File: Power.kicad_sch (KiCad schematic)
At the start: 48 parts, among them SW901 DP3T, U901 BQ24075, U902 TPS7A0533PDBV, U903 LP5907MFX-3.3

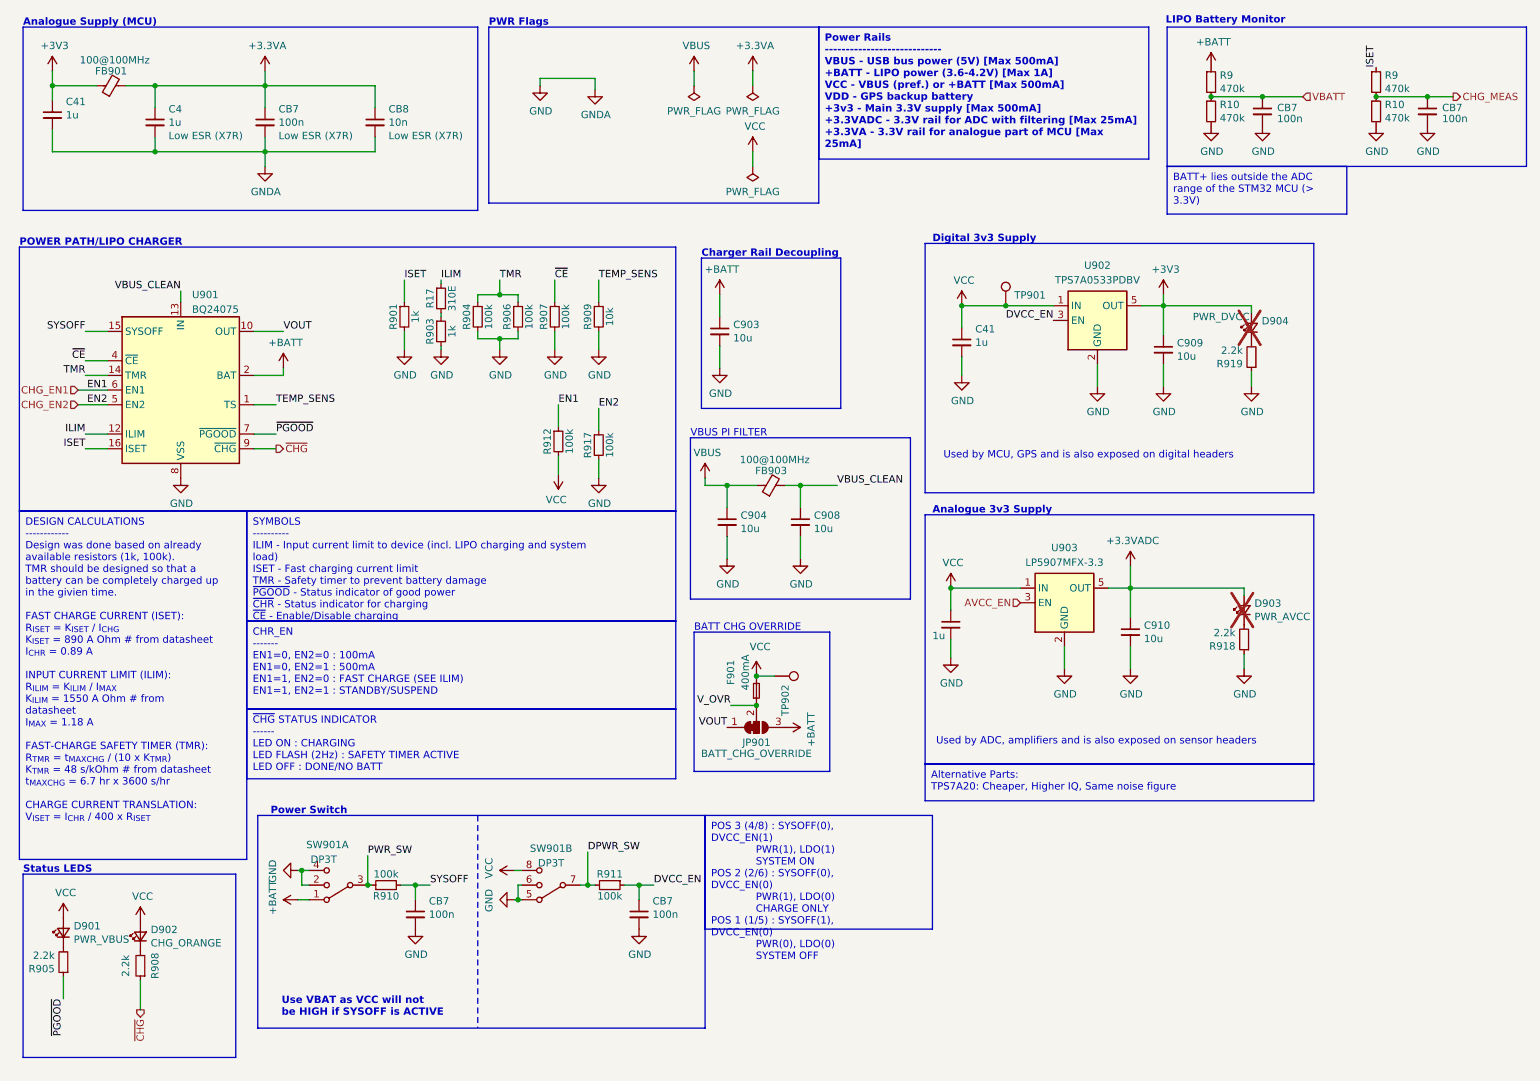
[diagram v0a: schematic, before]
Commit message: (sch) update annotations
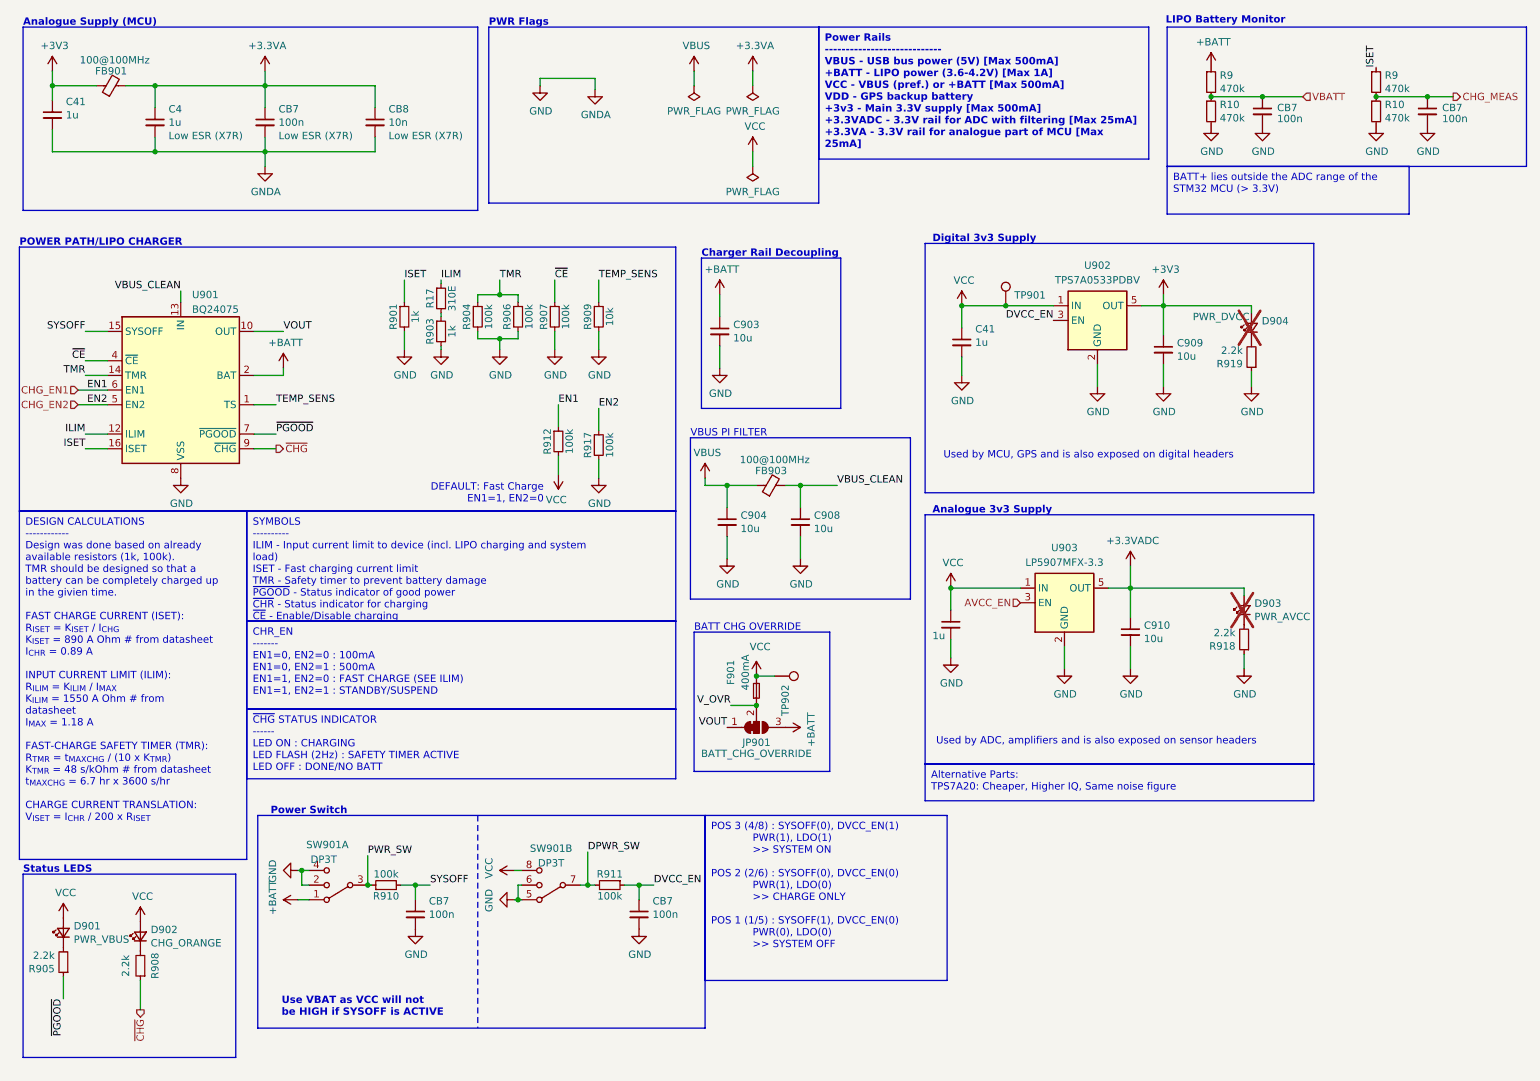
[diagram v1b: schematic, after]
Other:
- note added: "DEFAULT: Fast Charge EN1=1, EN2=0"
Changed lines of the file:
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@@
     (effects (font (size 1.27 1.27)) (justify left top))
   )
-  (text_box "DESIGN CALCULATIONS\n------------\nDesign was done based on already available resistors (1k, 100k).\nTMR should be designed so that a battery can be completely charged up in the givien time.\n\nFAST CHARGE CURRENT (ISET):\nR_{ISET} = K_{ISET} / I_{CHG}\nK_{ISET} = 890 A Ohm # from datasheet\nI_{CHR} = 0.89 A\n\nINPUT CURRENT LIMIT (ILIM):\nR_{ILIM} = K_{ILIM} / I_{MAX}\nK_{ILIM} = 1550 A Ohm # from datasheet\nI_{MAX} = 1.18 A\n\nFAST-CHARGE SAFETY TIMER (TMR):\nR_{TMR} = t_{MAXCHG} / (10 x K_{TMR})\nK_{TMR} = 48 s/kOhm # from datasheet\nt_{MAXCHG} = 6.7 hr x 3600 s/hr\n\nCHARGE CURRENT TRANSLATION:\nV_{ISET} = I_{CHR} / 400 x R_{ISET}"
+  (text_box "DESIGN CALCULATIONS\n------------\nDesign was done based on already available resistors (1k, 100k).\nTMR should be designed so that a battery can be completely charged up in the givien time.\n\nFAST CHARGE CURRENT (ISET):\nR_{ISET} = K_{ISET} / I_{CHG}\nK_{ISET} = 890 A Ohm # from datasheet\nI_{CHR} = 0.89 A\n\nINPUT CURRENT LIMIT (ILIM):\nR_{ILIM} = K_{ILIM} / I_{MAX}\nK_{ILIM} = 1550 A Ohm # from datasheet\nI_{MAX} = 1.18 A\n\nFAST-CHARGE SAFETY TIMER (TMR):\nR_{TMR} = t_{MAXCHG} / (10 x K_{TMR})\nK_{TMR} = 48 s/kOhm # from datasheet\nt_{MAXCHG} = 6.7 hr x 3600 s/hr\n\nCHARGE CURRENT TRANSLATION:\nV_{ISET} = I_{CHR} / 200 x R_{ISET}"
     (at 14.605 100.33 0) (size 39.37 60.325)
     (stroke (width 0) (type default))
@@
     (effects (font (size 1.27 1.27)) (justify left top))
   )
-  (text_box "POS 3 (4/8) : SYSOFF(0), DVCC_EN(1)\n			  PWR(1), LDO(1)\n			  SYSTEM ON\nPOS 2 (2/6) : SYSOFF(0), DVCC_EN(0)\n			  PWR(1), LDO(0)\n			  CHARGE ONLY\nPOS 1 (1/5) : SYSOFF(1), DVCC_EN(0)\n			  PWR(0), LDO(0)\n			  SYSTEM OFF"
-    (at 133.35 153.035 0) (size 39.37 19.685)
+  (text_box "POS 3 (4/8) : SYSOFF(0), DVCC_EN(1)\n			 PWR(1), LDO(1)\n			 >> SYSTEM ON\n\nPOS 2 (2/6) : SYSOFF(0), DVCC_EN(0)\n			 PWR(1), LDO(0)\n			 >> CHARGE ONLY\n\nPOS 1 (1/5) : SYSOFF(1), DVCC_EN(0)\n			 PWR(0), LDO(0)\n			 >> SYSTEM OFF"
+    (at 133.35 153.035 0) (size 41.91 28.575)
     (stroke (width 0) (type default))
     (fill (type none))
@@
   )
   (text_box "BATT+ lies outside the ADC range of the STM32 MCU (> 3.3V)"
-    (at 213.36 40.64 0) (size 31.115 8.255)
+    (at 213.36 40.64 0) (size 41.91 8.255)
     (stroke (width 0) (type default))
     (fill (type none))
@@
     (effects (font (size 1.27 1.27) (thickness 0.254) bold) (justify left bottom))
   )
+  (text "DEFAULT: Fast Charge\nEN1=1, EN2=0" (at 105.41 99.06 0)
+    (effects (font (size 1.27 1.27)) (justify right bottom))
+  )
   (text "Analogue 3v3 Supply" (at 172.72 100.965 0)
